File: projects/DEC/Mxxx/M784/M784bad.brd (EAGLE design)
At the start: 125.7 x 62.2 mm, 11 parts

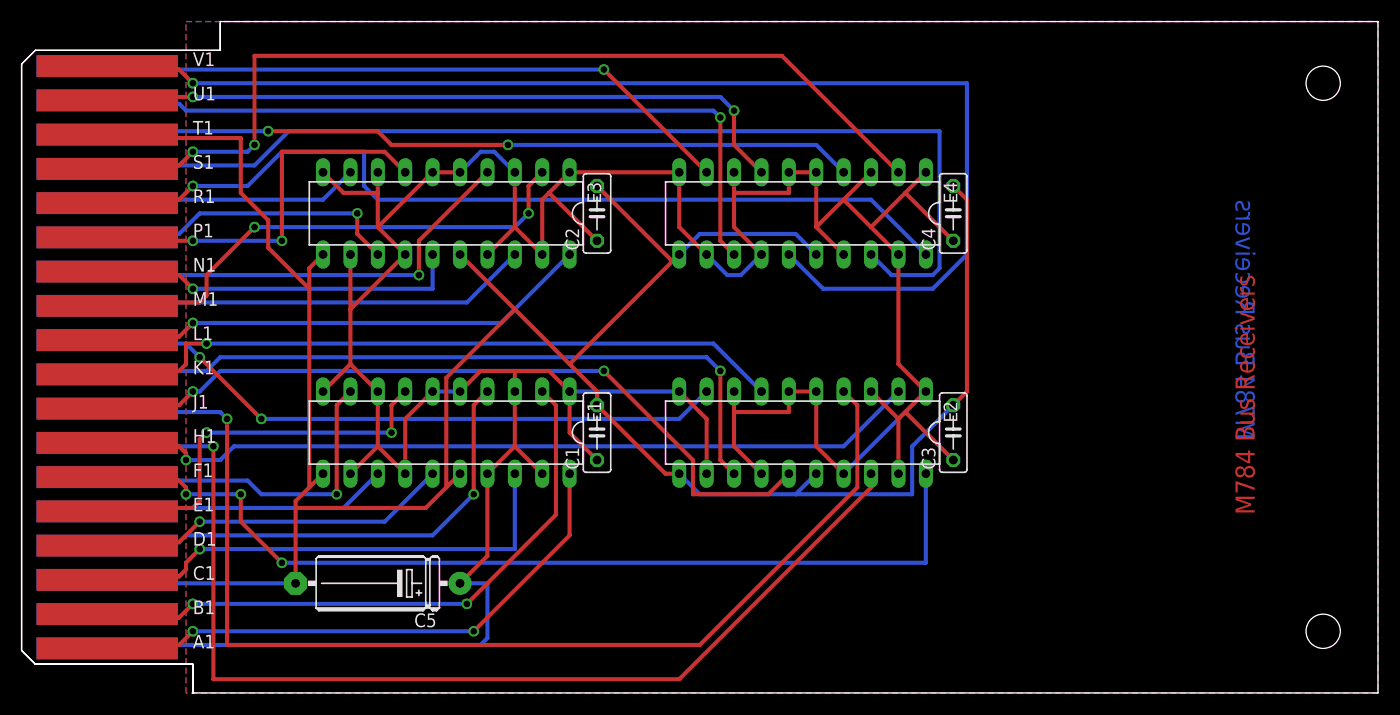
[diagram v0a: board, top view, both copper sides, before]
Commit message: Walk the project tree, making things pass current design rules.
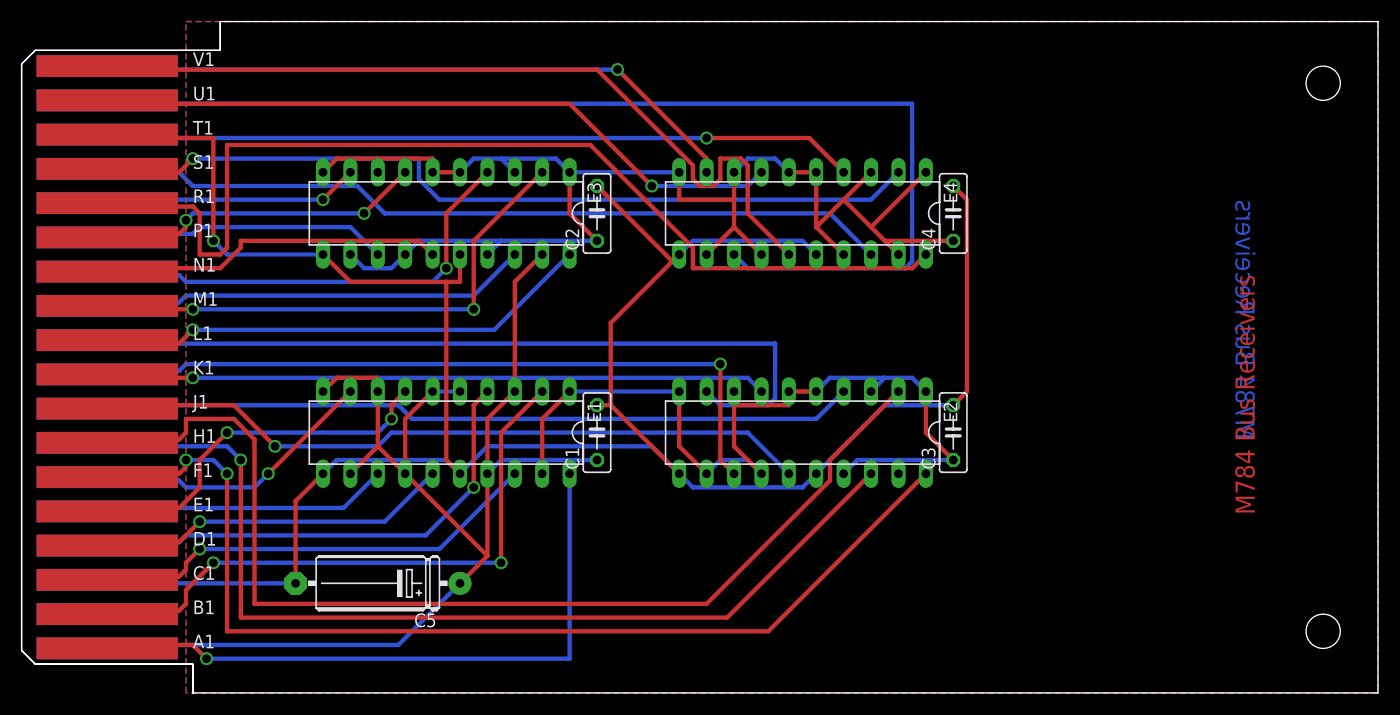
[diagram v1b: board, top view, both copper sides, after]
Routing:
- net N$12: track 115.4 -> 77.0 mm, vias 1 -> 0
- net N$21: track 106.3 -> 70.0 mm, vias 1 -> 0
- net N$10: track 70.7 -> 106.6 mm, vias 1 -> 0
- net N$14: track 98.7 -> 74.1 mm
- net N$23: track 77.0 -> 100.3 mm, vias 1 -> 0
- net VCC: track 362.9 -> 344.5 mm
- net N$18: track 59.6 -> 74.3 mm, vias 2 -> 0
- net N$15: track 83.7 -> 96.3 mm, vias 1 -> 0
- net N$22: track 101.2 -> 91.6 mm
- net GND: track 240.0 -> 230.7 mm, vias 0 -> 1
- net N$16: track 87.0 -> 77.7 mm, vias 2 -> 1
- net N$24: track 89.3 -> 98.1 mm, vias 3 -> 2
- net N$32: track 52.9 -> 60.7 mm, vias 2 -> 1
- net N$6: track 36.8 -> 30.5 mm
- net N$25: track 32.0 -> 26.6 mm
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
